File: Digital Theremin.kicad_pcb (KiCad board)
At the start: 2 copper layers, 95 x 55 mm, 55 parts, among them J1 Conn_01x02_Female, J2 AudioJack3, J3 USB_B_Micro, J4 Conn_01x03_Female, SW1 SW_Push, SW2 SW_Push, SW3 SW_SPDT, U1 AP2204K-3.0, U2 TDA2822, U3 NE555P, U4 NE555P, U5 STM32G051K8T6

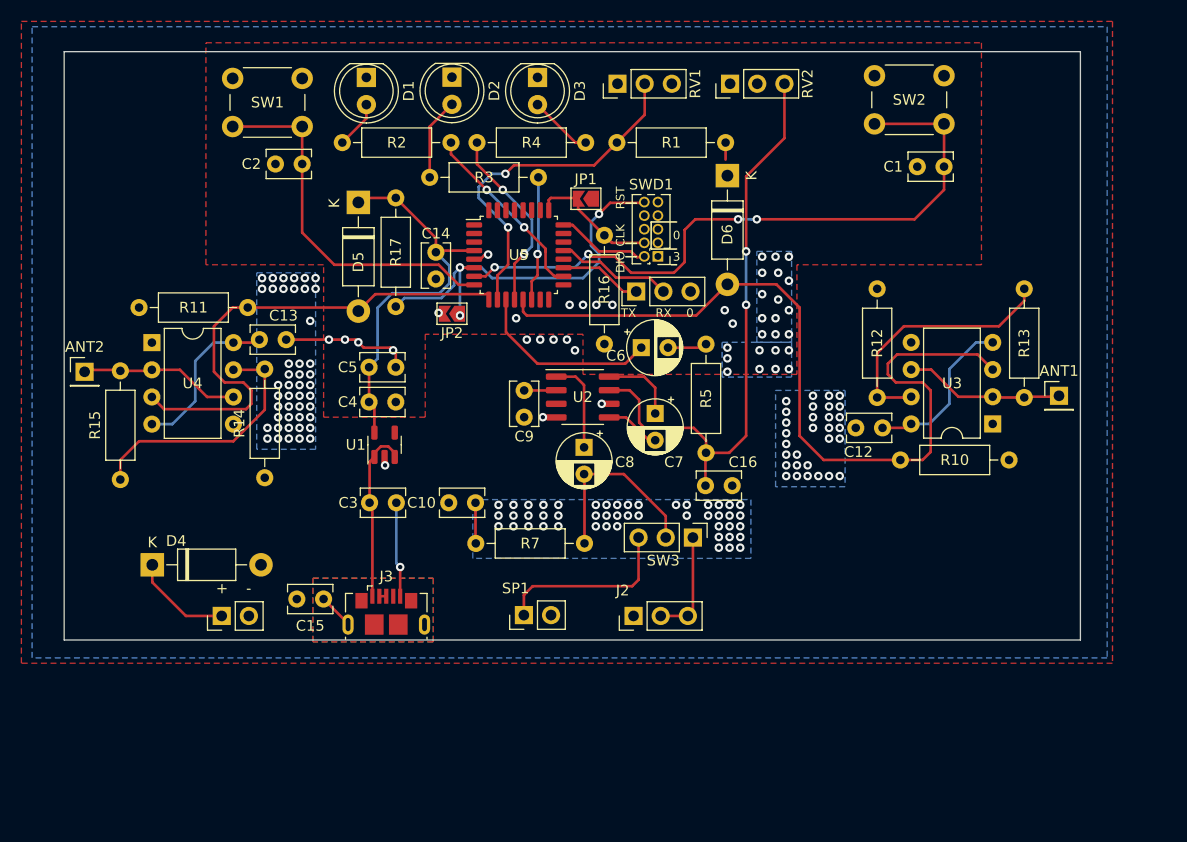
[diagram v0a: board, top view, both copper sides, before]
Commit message: Antenna mounts
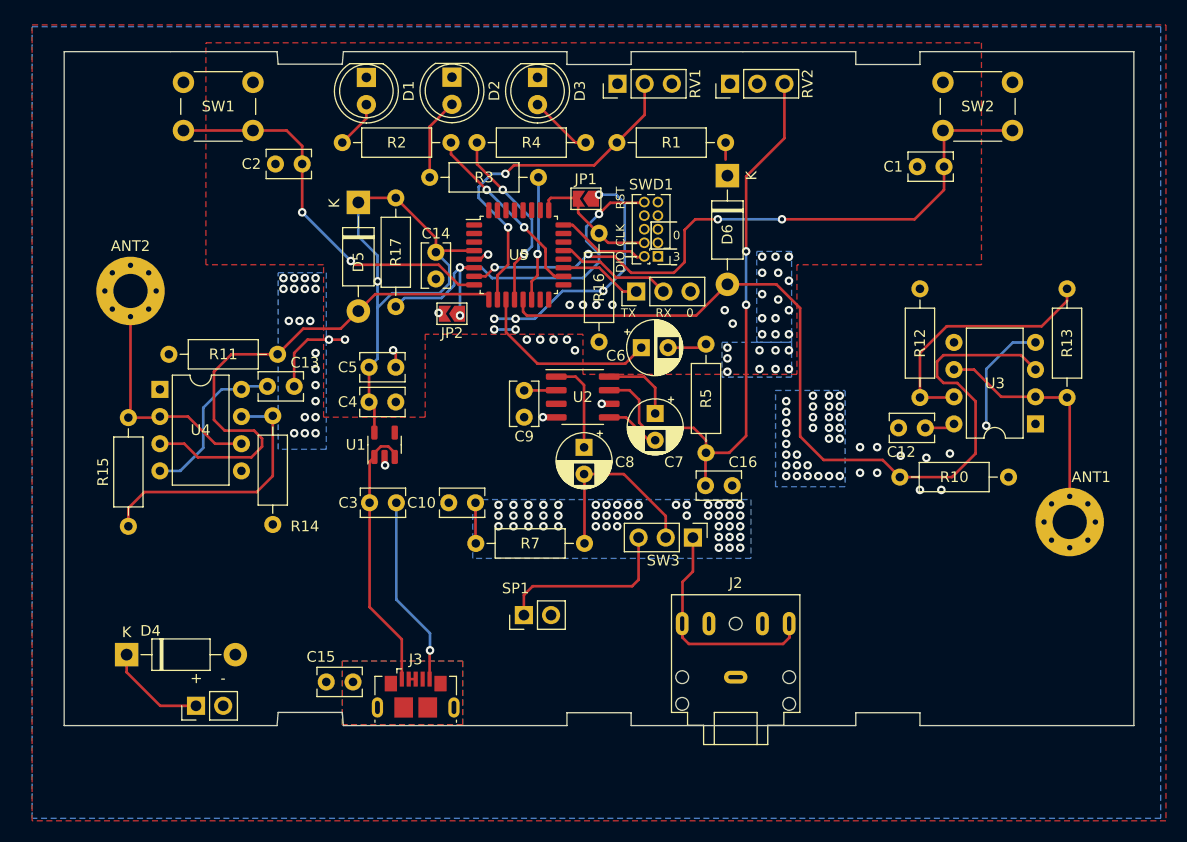
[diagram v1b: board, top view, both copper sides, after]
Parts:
- ANT1, ANT2: footprint Connector_PinHeader_2.54mm:PinHeader_1x01_P2.54mm_Vertical -> MountingHole:MountingHole_3.2mm_M3_Pad_Via
- J2: value AudioJack3 -> AudioJack3_Dual_Switch; footprint Connector_PinHeader_2.54mm:PinHeader_1x03_P2.54mm_Vertical -> Connector_Audio:Jack_3.5mm_CUI_SJ1-3525N_Horizontal
- moved ANT1 11.8 mm to (182.0, 105.8)
- moved J2 11.1 mm to (150.8, 120.3), turned to 0 degrees
- moved D4 8.74 mm to (93.8, 118.2)
- moved J1 8.74 mm to (100.3, 123.0)
- moved ANT2 8.69 mm to (94.2, 84.2)
- moved C15 8.22 mm to (115.0, 120.8)
- moved J3 8.22 mm to (120.9, 121.9)
- moved SW2 6.43 mm to (170.2, 64.7)
- moved R11 5.18 mm to (97.8, 90.1)
- moved SW1 4.61 mm to (99.2, 64.7)
- moved C13 4.43 mm to (107.0, 93.1)
- moved R14 4.43 mm to (107.5, 106.0)
- moved R15 4.43 mm to (94.0, 106.2)
- moved U4 4.43 mm to (97.0, 93.4)
- moved C12 4.00 mm to (168.5, 97.0)
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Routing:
- net +3V0: track 38.8 -> 75.1 mm, vias 24 -> 30
- net /Output: track 10.1 -> 21.9 mm
- net /Oscillators/Volume Antenna: track 15.2 -> 23.6 mm
- net /Oscillators/Pitch Antenna: track 15.2 -> 23.4 mm
- net +5V: track 60.0 -> 67.2 mm, vias 123 -> 108
- net GND: track 31.6 -> 38.5 mm, vias 21 -> 20
- net /Pitch Frequency: track 76.9 -> 81.1 mm
- net Net-(C15-Pad1): track 3.33 -> 0.00 mm
- net /Volume Frequency: track 47.4 -> 50.2 mm
- net /Function Button: track 34.5 -> 36.8 mm, vias 0 -> 2
- net Net-(R14-Pad2): track 24.0 -> 25.0 mm
- net /Calibrate Button: track 63.1 -> 62.6 mm
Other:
- board size 95 x 55 mm -> 100 x 63 mm
